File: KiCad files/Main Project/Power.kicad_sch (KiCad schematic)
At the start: 23 parts, among them J18 Conn_01x01, J19 Conn_01x01, U19 MCP73871-2CC

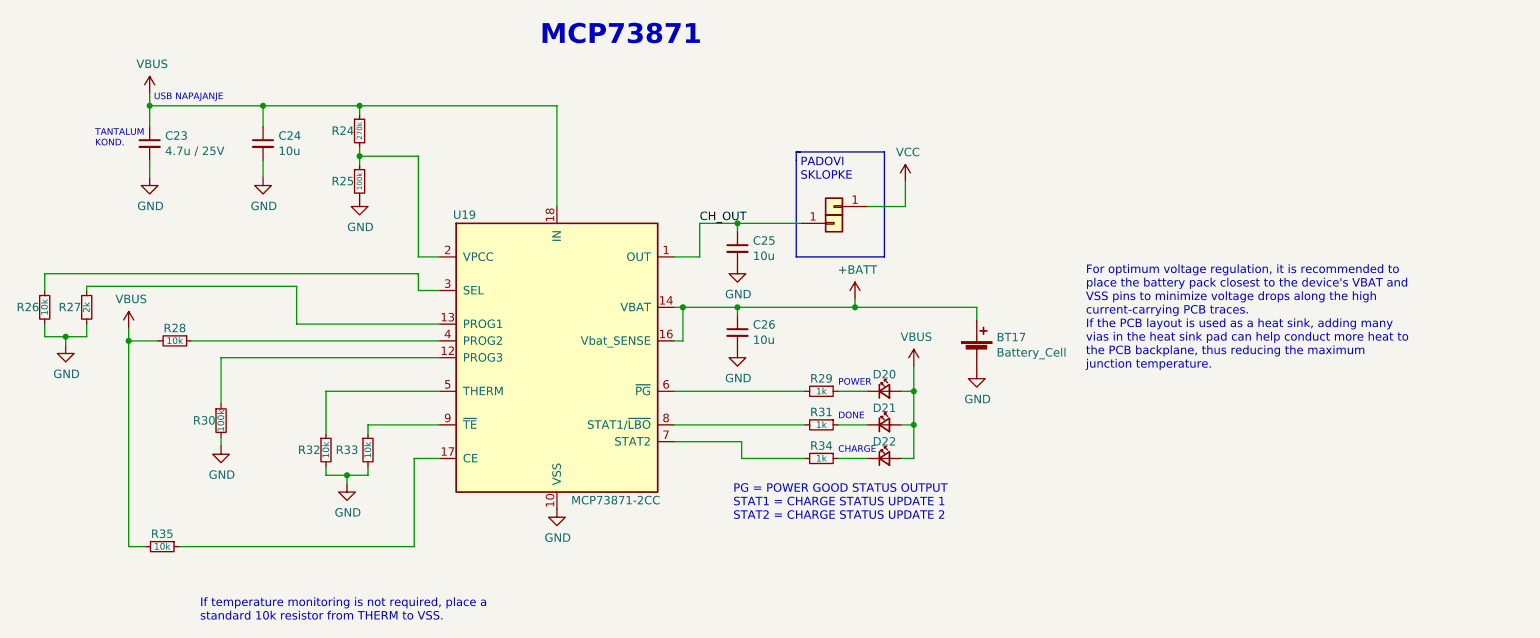
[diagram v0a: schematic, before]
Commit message: update
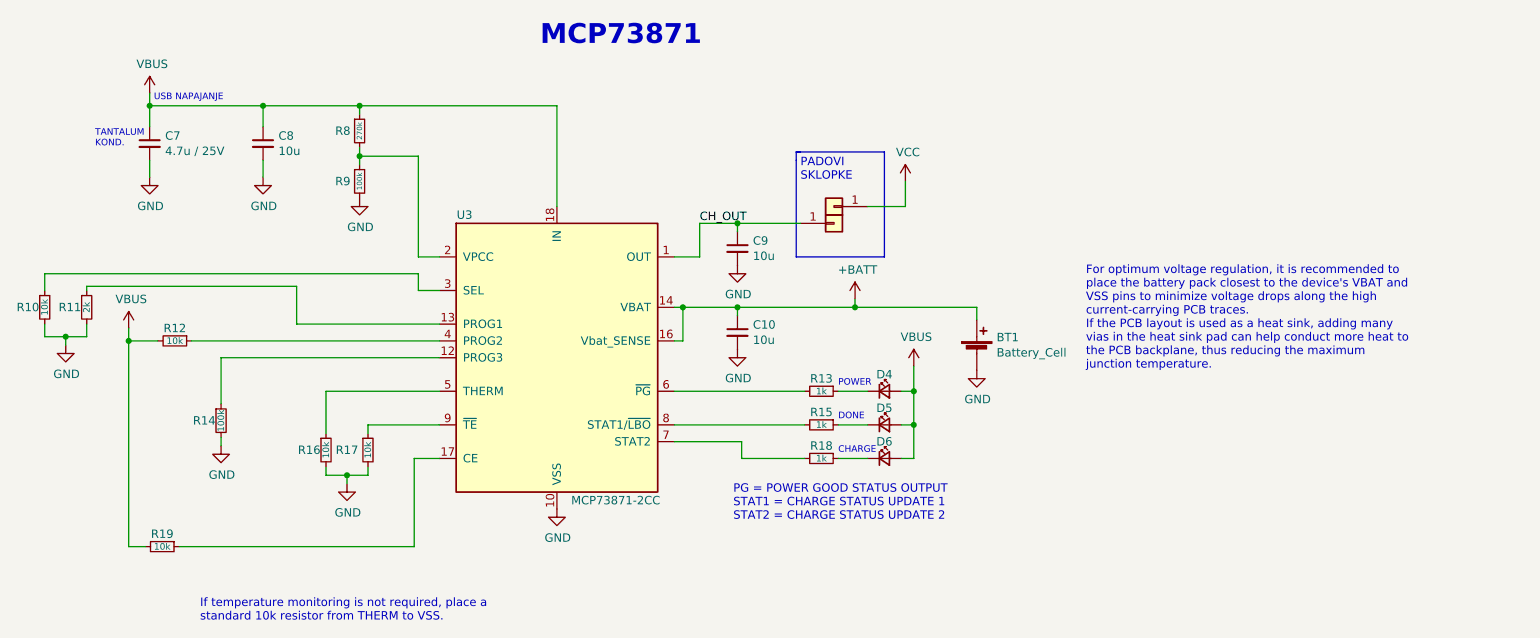
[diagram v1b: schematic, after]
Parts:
- renumbered BT17 to BT1, C26 to C10, C23 to C7, C24 to C8, C25 to C9, D20 to D4, D21 to D5, D22 to D6, J18 to J2, J19 to J3, R26 to R10, R27 to R11, R28 to R12, R29 to R13, R30 to R14, R31 to R15, R32 to R16, R33 to R17, R34 to R18, R35 to R19, R24 to R8, R25 to R9, U19 to U3

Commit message: update
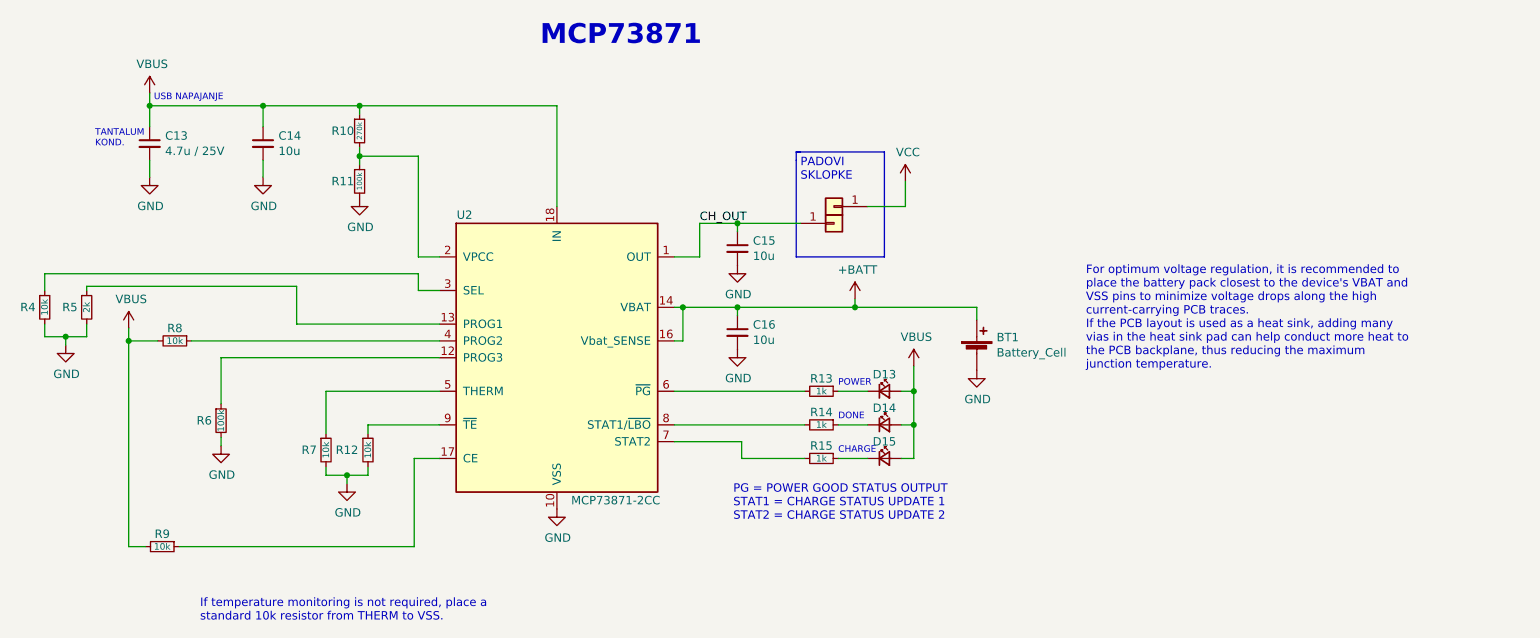
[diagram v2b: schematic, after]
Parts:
- renumbered C7 to C13, C8 to C14, C9 to C15, C10 to C16, D4 to D13, D5 to D14, D6 to D15, J2 to J21, J3 to J22, R8 to R10, R9 to R11, R17 to R12, R15 to R14, R18 to R15, R10 to R4, R11 to R5, R14 to R6, R16 to R7, R12 to R8, R19 to R9, U3 to U2

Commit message: shematic update
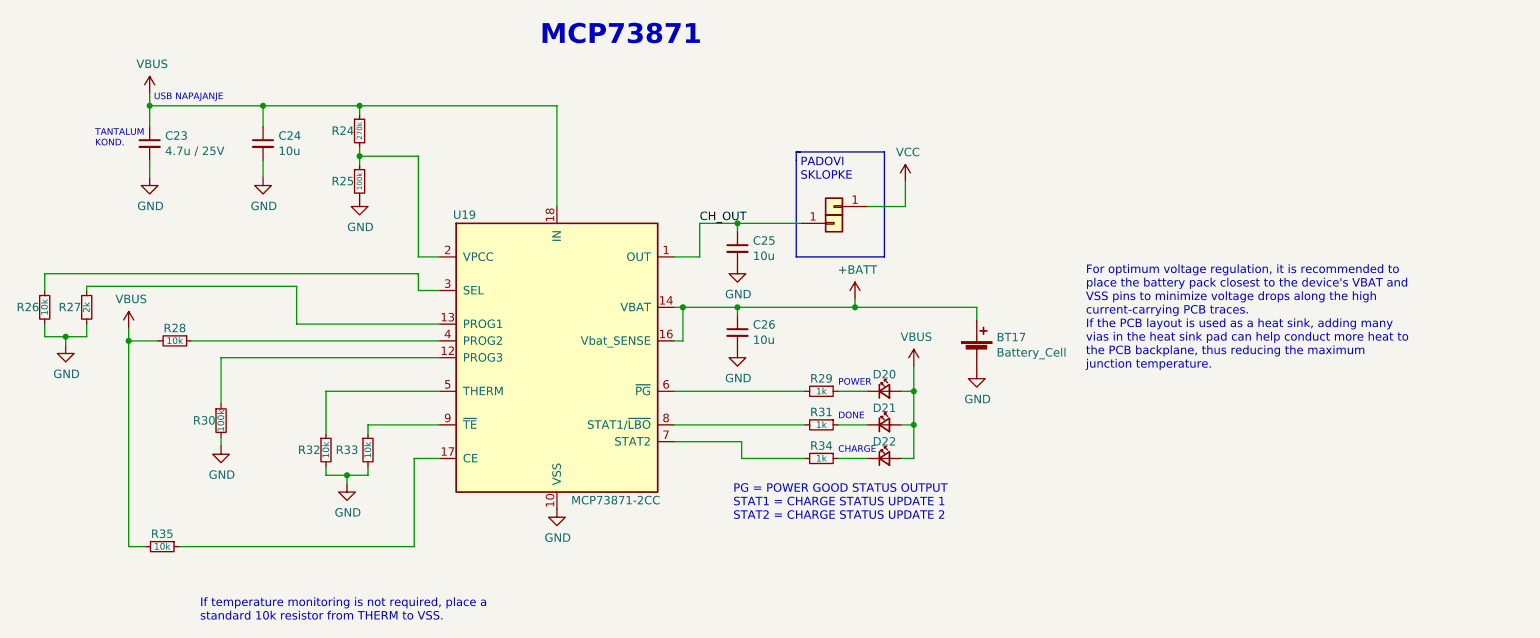
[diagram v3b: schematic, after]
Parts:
- renumbered BT1 to BT17, C13 to C23, C14 to C24, C15 to C25, C16 to C26, D13 to D20, D14 to D21, D15 to D22, J21 to J18, J22 to J19, R10 to R24, R11 to R25, R4 to R26, R5 to R27, R8 to R28, R13 to R29, R6 to R30, R14 to R31, R7 to R32, R12 to R33, R15 to R34, R9 to R35, U2 to U19
